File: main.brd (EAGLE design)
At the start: 24.5 x 25.1 mm, 36 parts, among them IC1 ATTINY13A-SSH, IC2 TP4056-42-ESOP8, IC3 LM27313XMFX_NOPB, T1A 2N4401, T1B NPN, X1 MINI-USB-UX60A-MB-5ST

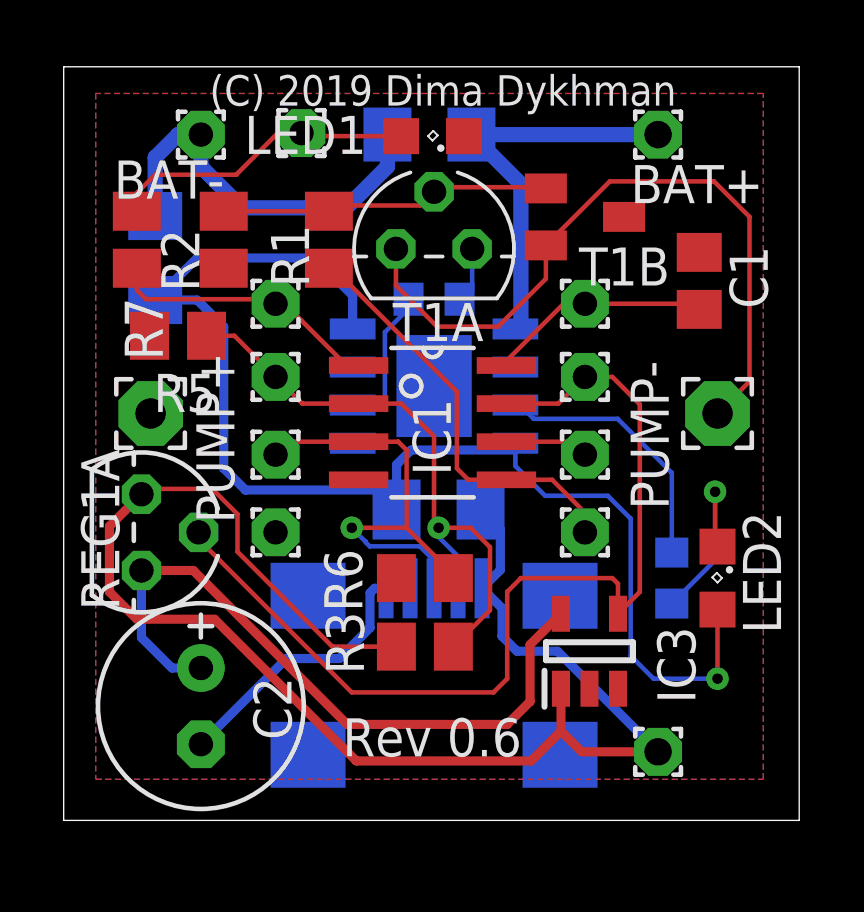
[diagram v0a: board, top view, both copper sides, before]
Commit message: new graphics
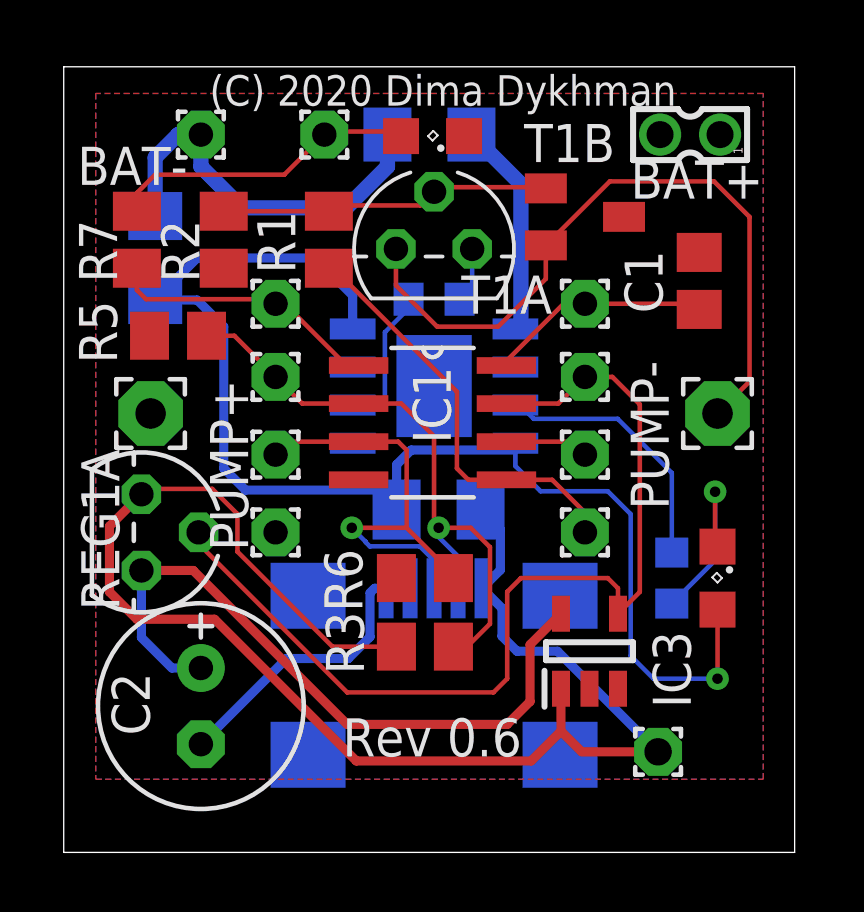
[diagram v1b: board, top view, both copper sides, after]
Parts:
- removed BAT+: (no value), wirepad:1,6/0,9
- added X2: 332-02, con-garry:332-02
- moved PAD1 0.76 mm to (9.60, 23.0)
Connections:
- net VCC: now also X2.1; no longer BAT+.1
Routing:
- net VCC: track 20.9 -> 14.7 mm
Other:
- board size 24.5 x 25.1 mm -> 24.4 x 26.2 mm
- board text added: "(C) 2020 Dima Dykhman"
- board text removed: "(C) 2019 Dima Dykhman"
